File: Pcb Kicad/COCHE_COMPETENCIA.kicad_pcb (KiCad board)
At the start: 2 copper layers, 95 x 62 mm, 39 parts, among them J1 BAT, J2 SWITCH, J4 M1, J5 M2, J6 SENSORES, Q1 2N3904, SW1 SW_Push, SW2 SW_Push, U2 ESP32-DEVKIT-V1, U3 DRV8833, U4 DRV8833, U5 AMS1117

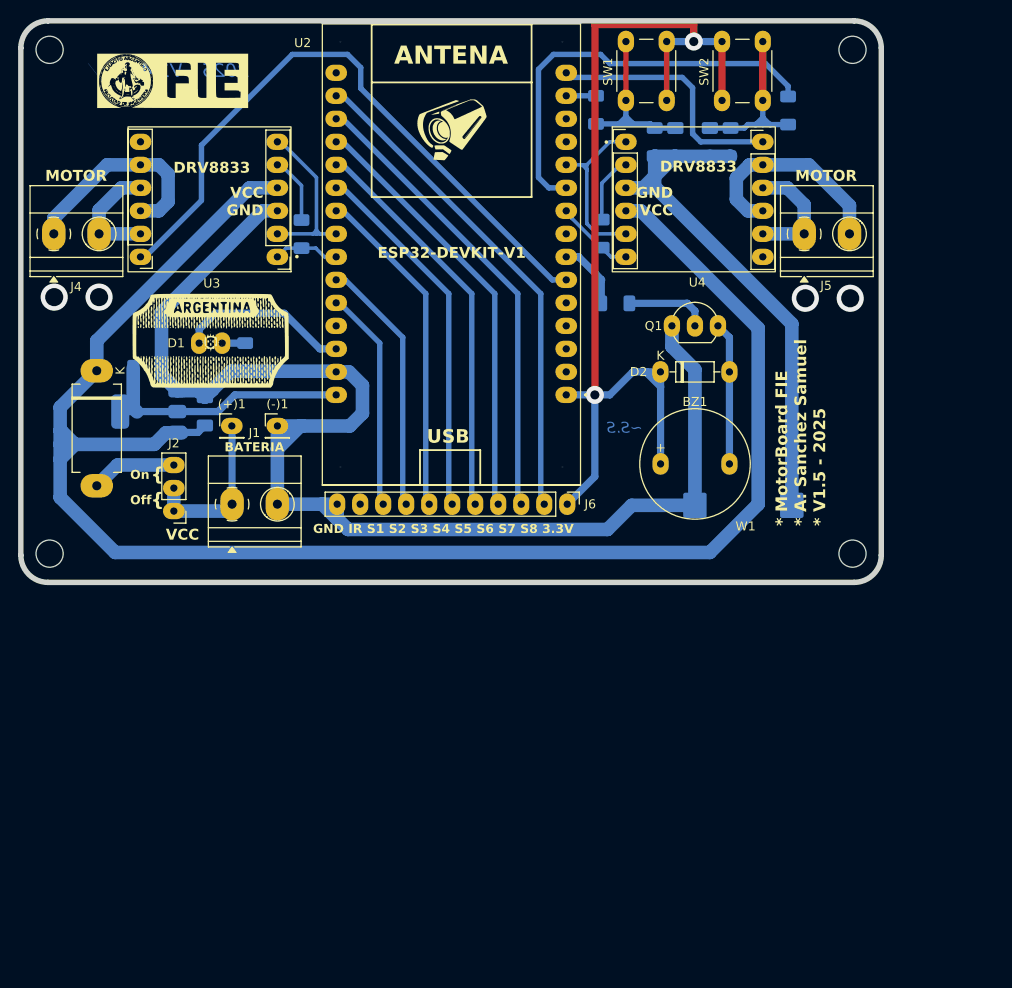
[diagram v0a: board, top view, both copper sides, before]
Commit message: V2.0 - Nueva version Seguidor De Linea
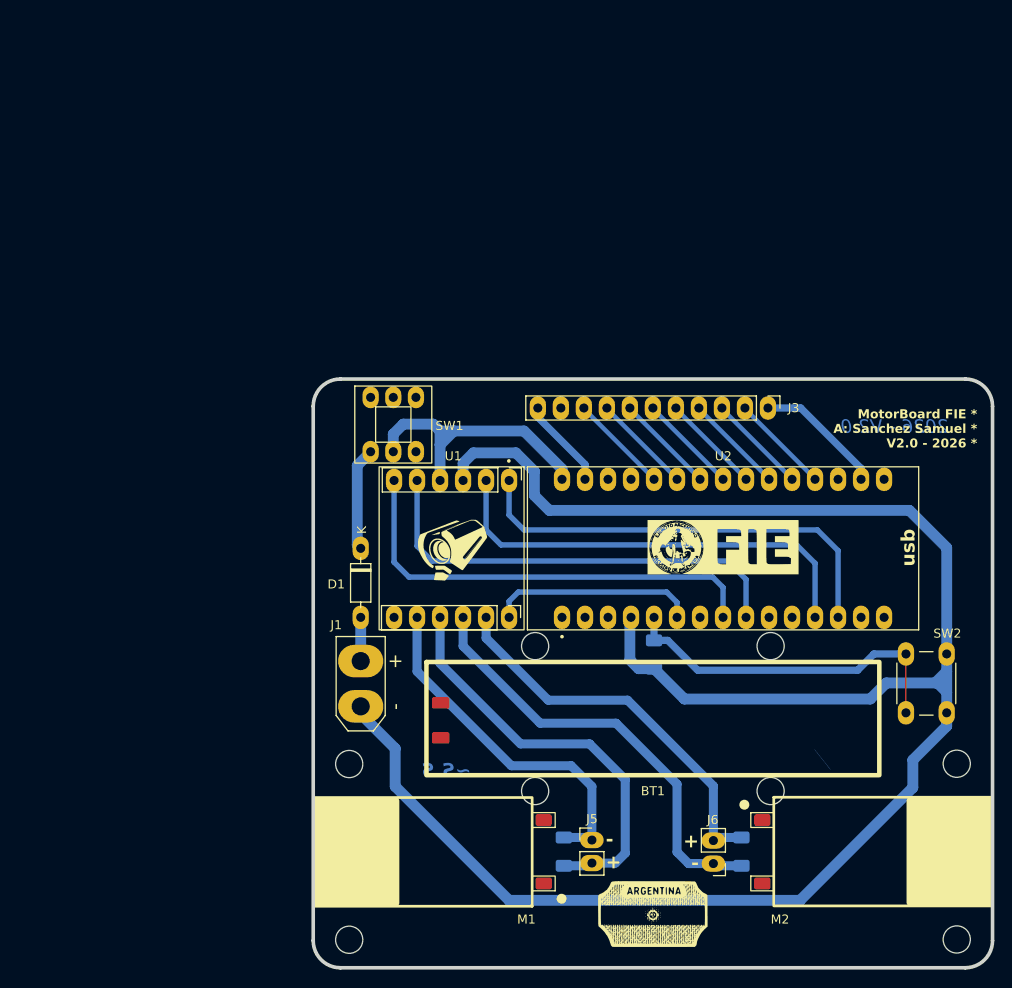
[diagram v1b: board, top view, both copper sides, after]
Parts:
- removed (+)1, (-)1: TestPoint, Connector_PinHeader_2.54mm:PinHeader_1x01_P2.54mm_Vertical
- removed BZ1: Buzzer, Buzzer_Beeper:MagneticBuzzer_ProSignal_ABI-009-RC
- removed C4: 100n, Capacitor_SMD:C_1206_3216Metric_Pad1.33x1.80mm_HandSolder
- removed D2: 1N4148, Diode_THT:D_DO-35_SOD27_P7.62mm_Horizontal
- removed D3: 1N5822, Diode_THT:D_DO-201AD_P12.70mm_Horizontal
- removed H1, H2, H3, H4: MountingHole, MountingHole:MountingHole_3mm
- removed J2: SWITCH, Connector_PinHeader_2.54mm:PinHeader_1x03_P2.54mm_Vertical
- removed J4: M1, TerminalBlock_Phoenix:TerminalBlock_Phoenix_MKDS-1,5-2_1x02_P5.00mm_Horizontal
- removed Q1: 2N3904, Package_TO_SOT_THT:TO-92_Inline_Wide
- removed R2, R3: 10k, Resistor_SMD:R_1206_3216Metric_Pad1.30x1.75mm_HandSolder
- removed R4: 220, Resistor_SMD:R_1206_3216Metric_Pad1.30x1.75mm_HandSolder
- removed R5, R6: 0, Resistor_SMD:R_1206_3216Metric_Pad1.30x1.75mm_HandSolder
- removed R7: 1k, Resistor_SMD:R_1206_3216Metric_Pad1.30x1.75mm_HandSolder
- removed R8, R9: 100, Resistor_SMD:R_1206_3216Metric_Pad1.30x1.75mm_HandSolder
- removed U3, U4: DRV8833, DRV8833:DRV8833
- removed U5: AMS1117, Package_TO_SOT_SMD:SOT-223-3_TabPin2
- removed W1: 5104, JUMPLER 5104:KEYSTONE_5104
- added BT1: 2S 70C 250mAH, Bateria_9S:Bateria_Lado, F.Cu at (167.4, 102.7)
- added J3: SENSORES, Connector_PinHeader_2.54mm:PinHeader_1x11_P2.54mm_Vertical, F.Cu at (180.1, 68.4)
- added M1: Pololu DC, PololuLibrary:pololu, F.Cu at (154.1, 117.4)
- added M2: Pololu DC, PololuLibrary:pololu, F.Cu at (180.8, 117.4)
- added U1: DRV8833, DRV8833:DRV8833, F.Cu at (135.3, 84.3)
- C2: value 1u -> 100n
- D1: value LED_RED -> D_Schottky; footprint LED_THT:LED_D5.0mm -> Diode_THT:D_DO-35_SOD27_P7.62mm_Horizontal
- J1: footprint TerminalBlock_Phoenix:TerminalBlock_Phoenix_MKDS-1,5-2_1x02_P5.00mm_Horizontal -> Connector_AMASS:AMASS_XT30UPB-M_1x02_P5.0mm_Vertical
- J5: value M2 -> M1; footprint TerminalBlock_Phoenix:TerminalBlock_Phoenix_MKDS-1,5-2_1x02_P5.00mm_Horizontal -> Connector_PinHeader_2.54mm:PinHeader_1x02_P2.54mm_Vertical
- J6: value SENSORES -> M2; footprint Connector_PinHeader_2.54mm:PinHeader_1x11_P2.54mm_Vertical -> Connector_PinHeader_2.54mm:PinHeader_1x02_P2.54mm_Vertical
- SW1: value SW_Push -> ON/OFF; footprint Button_Switch_THT:SW_PUSH_6mm_H5mm -> switch6P:SWITCH_6PINS
- SW2: value SW_Push -> SW_RUN
- U2: value ESP32-DEVKIT-V1 -> ARDUINO_NANO; footprint ESP32-DEVKIT-V1:MODULE_ESP32_DEVKIT_V1 -> Arduino NANO:MODULE_ARDUINO_NANO
- moved G*** 110.3 mm to (188.5, 107.1)
- moved G*** 79.9 mm to (167.4, 124.3)
- moved G*** 79.6 mm to (175.2, 83.7)
- moved C3 78.7 mm to (177.2, 117.4)
- moved J5 70.9 mm to (160.7, 116.1)
- moved SW2 70.6 mm to (195.4, 102.0)
- moved C2 70.5 mm to (157.6, 117.4), turned to -90 degrees
- moved C1 56.4 mm to (167.6, 95.6), turned to -90 degrees
- moved SW1 52.0 mm to (138.8, 70.2), turned to 0 degrees
- moved G*** 46.4 mm to (145.2, 84.1)
- moved U2 44.2 mm to (175.2, 83.9), turned to 90 degrees
- moved J6 42.8 mm to (174.1, 118.7), turned to 180 degrees
- moved D1 27.3 mm to (135.2, 83.9), turned to -90 degrees
- moved J1 26.5 mm to (135.2, 101.3), turned to 90 degrees
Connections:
- C1 pad 1: VCC -> /SW1
- C1 pad 2: GND -> GND_BAT
- C2 pad 1: +5V -> /OUT1-
- C2 pad 2: GND -> /OUT1+
- C3 pad 1: Net-(C3-Pad1) -> /OUT2+
- C3 pad 2: GND -> /OUT2-
- D1 pad 2: /LED_LARGADA -> /BAT+
- J1 pad 1: Net-(J1-Pin_1) -> GND_BAT
- J1 pad 2: GND -> /BAT+
- J5 pad 1: Net-(J5-Pin_1) -> /OUT1-
- J5 pad 2: Net-(J5-Pin_2) -> /OUT1+
- J6 pad 1: +3.3V -> /OUT2-
- J6 pad 2: /S8 -> /OUT2+
- SW1 pad 1: +3.3V -> unconnected-(SW1-A-Pad1)
- SW1 pad 2: Net-(C3-Pad1) -> VCC
- SW2 pad 1: +3.3V -> /SW1
- SW2 pad 2: Net-(C4-Pad1) -> GND_BAT
- U2 pad 1: +3.3V -> /TX
- U2 pad 10: /SW2 -> unconnected-(U2-D7-Pad10)
- U2 pad 11: /IN_M2_A -> unconnected-(U2-D8-Pad11)
- U2 pad 12: unconnected-(U2-RX0-Pad12) -> /IN_M1_B
- U2 pad 13: unconnected-(U2-TX0-Pad13) -> /IN_M1_A
- U2 pad 14: /SW1 -> unconnected-(U2-D11/MOSI-Pad14)
- U2 pad 15: /SLEEP_M2 -> unconnected-(U2-D12/MISO-Pad15)
- U2 pad 16: unconnected-(U2-EN-Pad16) -> /LED_LARGADA
- U2 pad 17: /S8 -> +3.3V
- U2 pad 18: /S7 -> unconnected-(U2-AREF-Pad18)
- U2 pad 19: /S6 -> /S8
- U2 pad 2: GND -> /RX
- U2 pad 20: /S5 -> /S7
- U2 pad 21: /S4 -> /S6
- U2 pad 22: /S3 -> /S5
- U2 pad 23: /IN_M1_B -> /S4
- U2 pad 24: /IN_M1_A -> /S3
- U2 pad 27: unconnected-(U2-D12-Pad27) -> +5.0V
- U2 pad 28: /LED_LARGADA -> unconnected-(U2-RESET-Pad28)
- U2 pad 30: +5V -> VCC
- U2 pad 4: unconnected-(U2-D2-Pad4) -> GND_BAT
- U2 pad 5: unconnected-(U2-D4-Pad5) -> /SW1
- U2 pad 6: /SLEEP_M1 -> /SLEEP
- U2 pad 7: /BUZZER -> unconnected-(U2-D4-Pad7)
- U2 pad 8: unconnected-(U2-D5-Pad8) -> /IN_M2_B
- U2 pad 9: /IN_M2_B -> /IN_M2_A
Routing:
- net GND_BAT: track 0.00 -> 212.1 mm
- net GND: track 210.8 -> 10.0 mm
- net VCC: track 189.0 -> 31.8 mm
- net +3.3V: track 110.3 -> 14.3 mm, vias 2 -> 0
- net /SLEEP_M1: track 71.5 -> 0.00 mm
- net /OUT2-: track 0.00 -> 48.0 mm
- net /OUT1+: track 0.00 -> 46.3 mm
- net /SW2: track 46.3 -> 0.00 mm
- net /S8: track 55.0 -> 11.1 mm
- net /OUT2+: track 0.00 -> 43.4 mm
- net /IN_M1_A: track 7.29 -> 49.1 mm
- net /IN_M2_B: track 8.89 -> 49.8 mm
- net /S7: track 51.4 -> 11.1 mm
- net /OUT1-: track 0.00 -> 39.7 mm
- net /S6: track 47.9 -> 11.1 mm
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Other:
- board size 95 x 62 mm -> 75 x 65 mm
- board text added: "+ -"
- board text added: "2026 - V2.0"
- board text added: "MotorBoard FIE * A: Sanchez Samuel * V2.0 - 2026 *"
- board text added: "usb"
- board text removed: "* MotorBoard FIE * A: Sanchez Samuel * V1.5 - 2025"
- board text removed: "2025 - V1.4"
- board text removed: "ANTENA"
- board text removed: "BATERIA"
- board text removed: "DRV8833"
- board text removed: "ESP32-DEVKIT-V1"
- board text removed: "GND IR S1 S2 S3 S4 S5 S6 S7 S8 3.3V"
- board text removed: "GND VCC"
- board text removed: "MOTOR"
- board text removed: "Off"
- board text removed: "On"
- board text removed: "USB"
- board text removed: "VCC"
- board text removed: "VCC GND"
- board text removed: "{"
